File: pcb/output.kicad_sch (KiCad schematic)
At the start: 12 parts, among them J2 Lights, J3 Current Conn, Q1 MOSFET, Q2 MOSFET, Q3 N-MOS, U2 L9110H, U4 BCR430

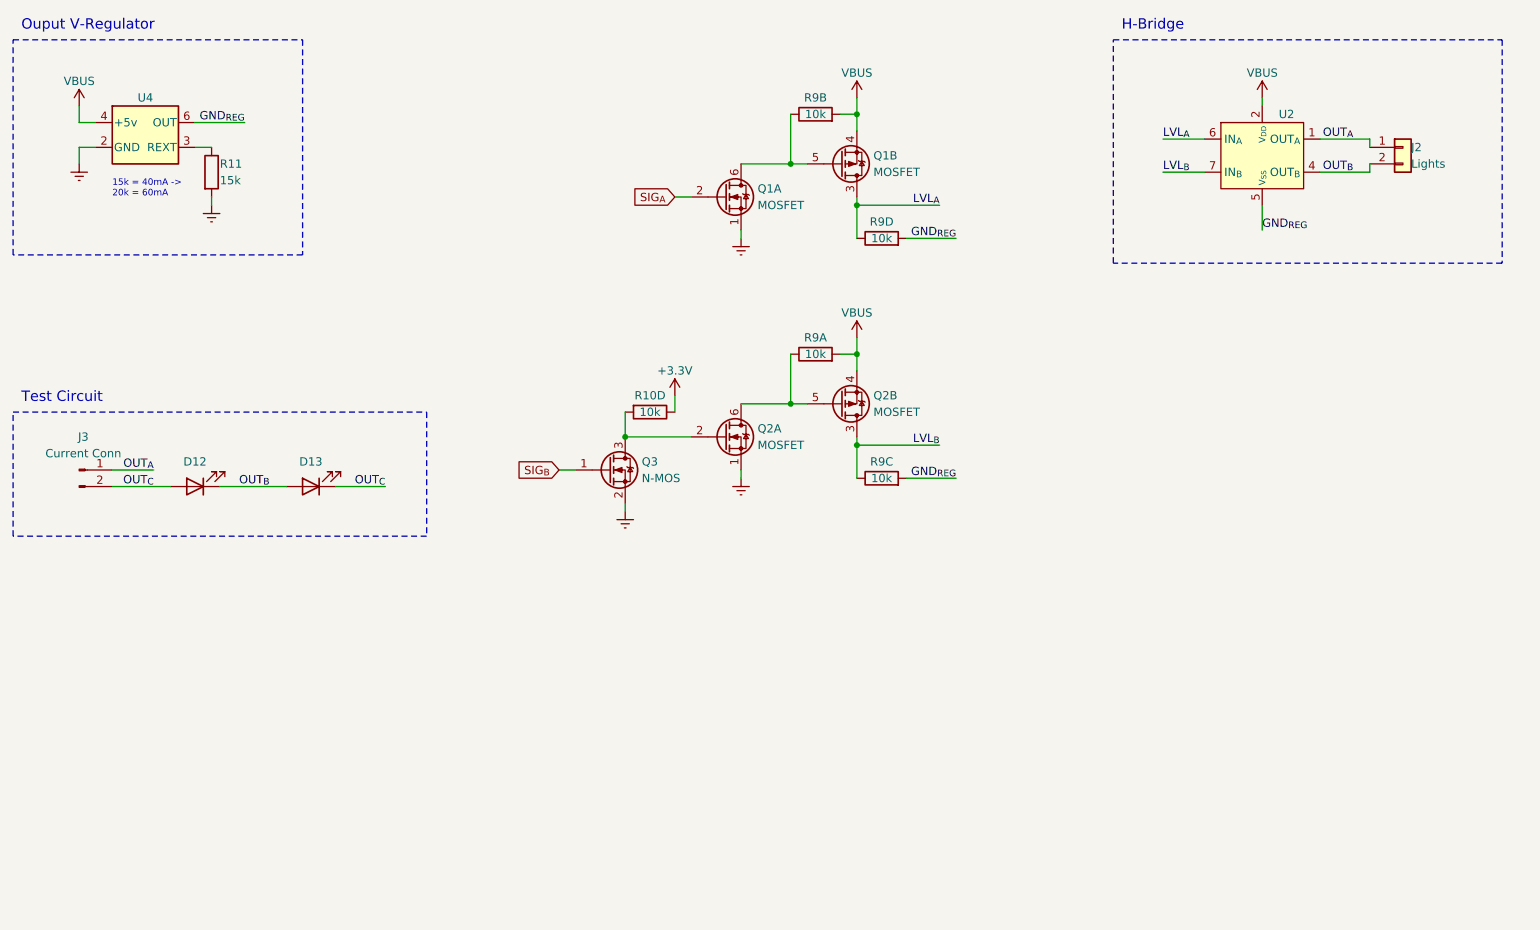
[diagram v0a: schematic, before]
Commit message: pcb updates
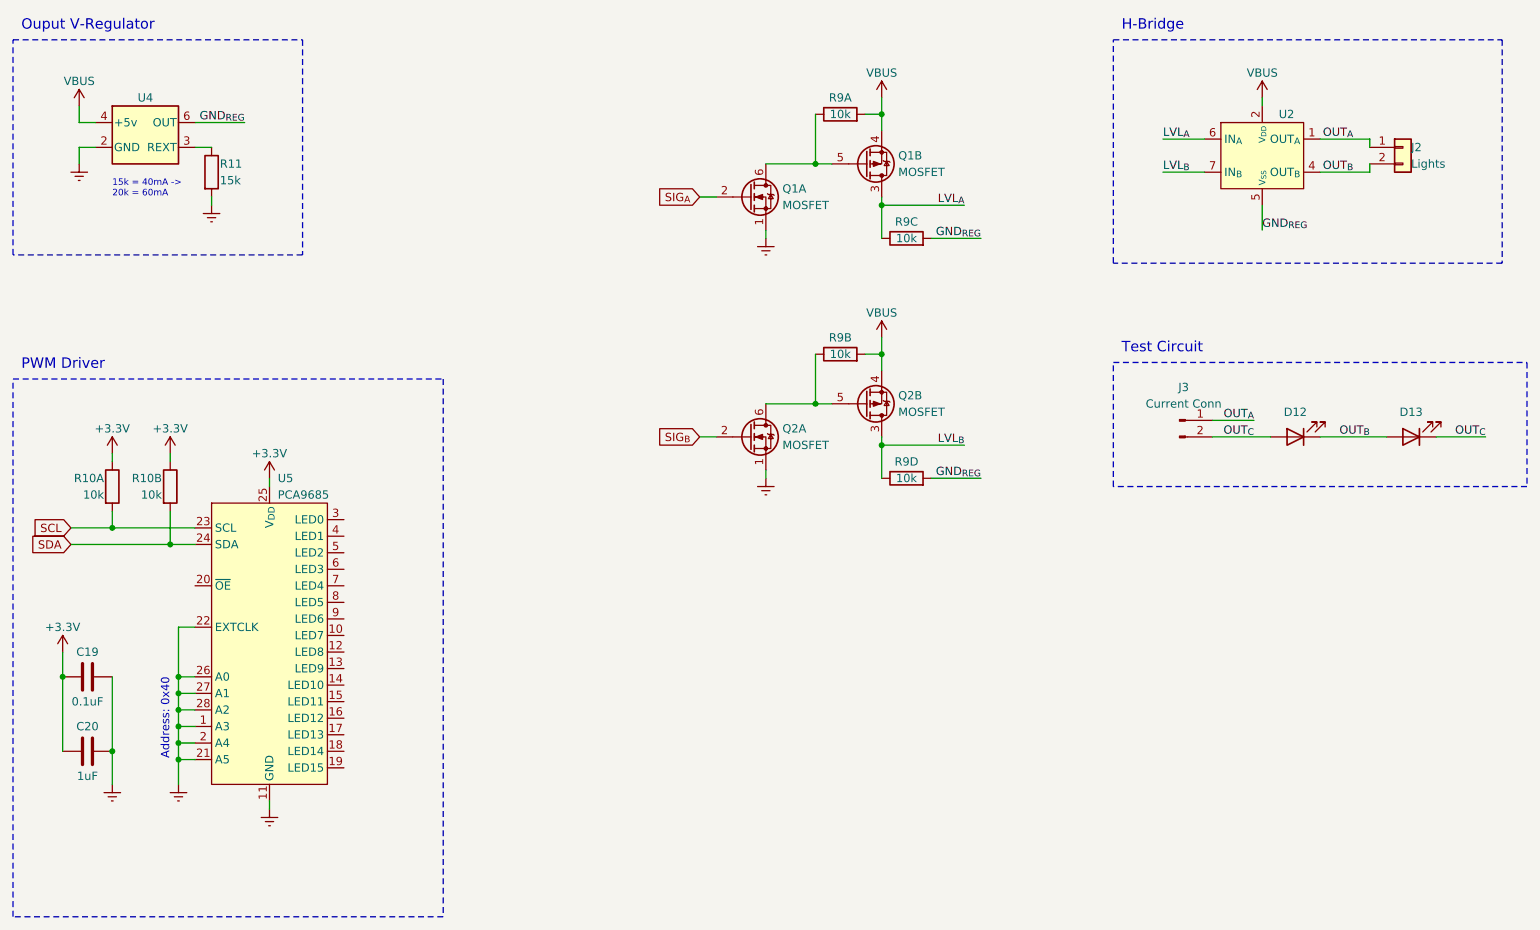
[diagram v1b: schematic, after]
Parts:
- removed Q3: N-MOS, _custom:Transistor_SOT-323, symbol _custom:MOSFET_N-Ch
- removed R10: 10k, _custom:R_Array_4x1206_Convex, symbol _custom:Resistor_Array_4x
- added C19: 0.1uF, _custom:CAP_0402_HandSolder, symbol _custom:CAP_Standard
- added C20: 1uF, _custom:CAP_0603_HandSolder, symbol _custom:CAP_Standard
- added R10: 10k, _custom:R_Array_4x1206_Convex, symbol _custom:Resistor_Array_4x
- added U5: PCA9685, _custom:GenericIC_VQFN-28-EP-6x6mm, symbol _custom:PCA9685
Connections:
- net +3.3V: now also C19.1, C20.1, R10.1, R10.3, U5.25 (V_{DD})
- net GNDREF: now also C19.2, C20.2, U5.1 (A3), U5.11 (GND), U5.2 (A4), U5.21 (A5), U5.22 (EXTCLK), U5.26 (A0), U5.27 (A1), U5.28 (A2)
- net LVL_{A}: now also R9.5; no longer R9.7
- net LVL_{B}: now also R9.7; no longer R9.5
- net SIG_{B}: now also Q2.2 (G_{A})
- net at Q2.5 (G_{B}), Q2.6 (D_{A}): now also R9.3; no longer R9.1
- net at Q1.5 (G_{B}), Q1.6 (D_{A}): now also R9.1; no longer R9.3
- new net SCL: R10.2, U5.23 (SCL)
- new net SDA: R10.4, U5.24 (SDA)
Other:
- note added: "Address: 0x40"
- note added: "PWM Driver"
- moved on the sheet: D12, D13, J3, Q1A, Q1B, Q2A, Q2B, R9A, R9B, R9C, R9D
